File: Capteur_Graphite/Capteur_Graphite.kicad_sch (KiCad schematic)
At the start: 21 parts, among them J1 Power, J2 Digital/PWM, J3 Analog, J4 Digital/PWM, U1 LTC1050ACN8_PBF, U2 MCP41050

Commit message: Clear PCB
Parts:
- C3, C4: footprint Capacitor_THT:C_Rect_L7.5mm_W6.5mm_P5.00mm -> Capacitor_THT:C_Rect_L7.0mm_W4.5mm_P5.00mm
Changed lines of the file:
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@@
 			)
 		)
-		(property "Footprint" "Capacitor_THT:C_Rect_L7.5mm_W6.5mm_P5.00mm"
+		(property "Footprint" "Capacitor_THT:C_Rect_L7.0mm_W4.5mm_P5.00mm"
 			(at 135.5852 40.64 0)
 			(effects
@@
 			)
 		)
-		(property "Footprint" "Capacitor_THT:C_Rect_L7.5mm_W6.5mm_P5.00mm"
+		(property "Footprint" "Capacitor_THT:C_Rect_L7.0mm_W4.5mm_P5.00mm"
 			(at 172.4152 96.52 0)
 			(effects

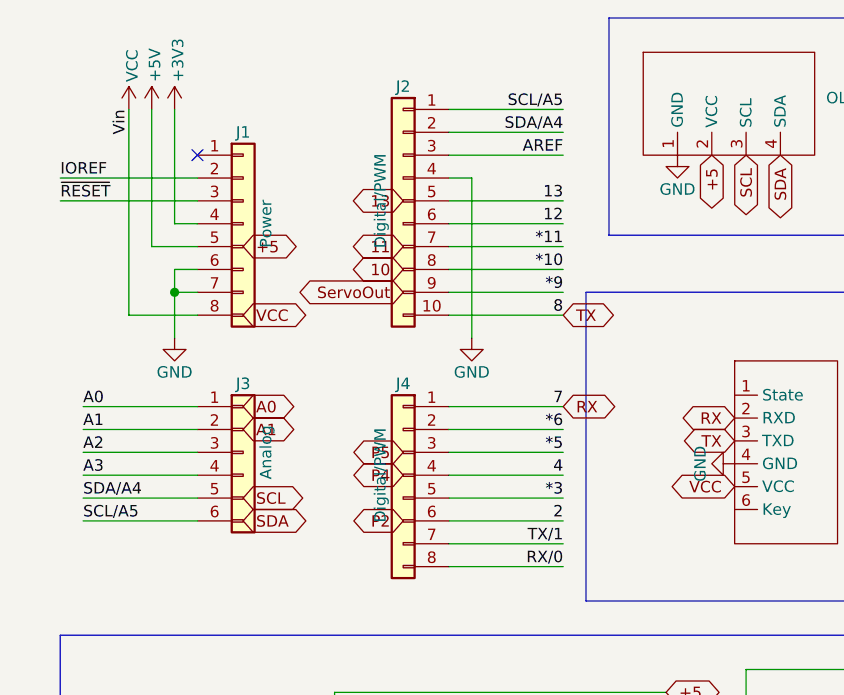
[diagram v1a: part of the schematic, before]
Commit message: Schematique propre
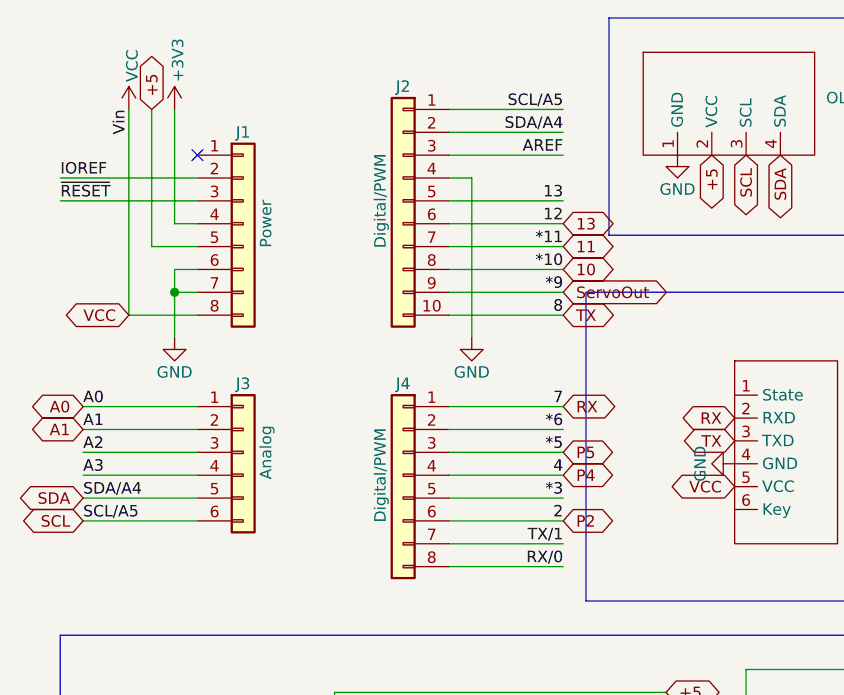
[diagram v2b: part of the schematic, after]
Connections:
- net *10 is gone; now on net 10: J2.8 (Pin_8)
- net *11 is gone; now on net 11: J2.7 (Pin_7)
- net *5 is gone; now on net P5: J4.3 (Pin_3)
- net *9 is gone; now on net ServoOut: J2.9 (Pin_9)
- net +5V is gone; now on net +5: J1.5 (Pin_5)
- net 12 is gone; now on net 13: J2.6 (Pin_6)
- net 2 is gone; now on net P2: J4.6 (Pin_6)
- net 4 is gone; now on net P4: J4.4 (Pin_4)
- net SCL/A5 is gone; now on net SCL: J2.1 (Pin_1), J3.6 (Pin_6)
- net SDA/A4 is gone; now on net SDA: J2.2 (Pin_2), J3.5 (Pin_5)
